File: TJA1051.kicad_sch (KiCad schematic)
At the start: 9 parts, among them U1 BMI088

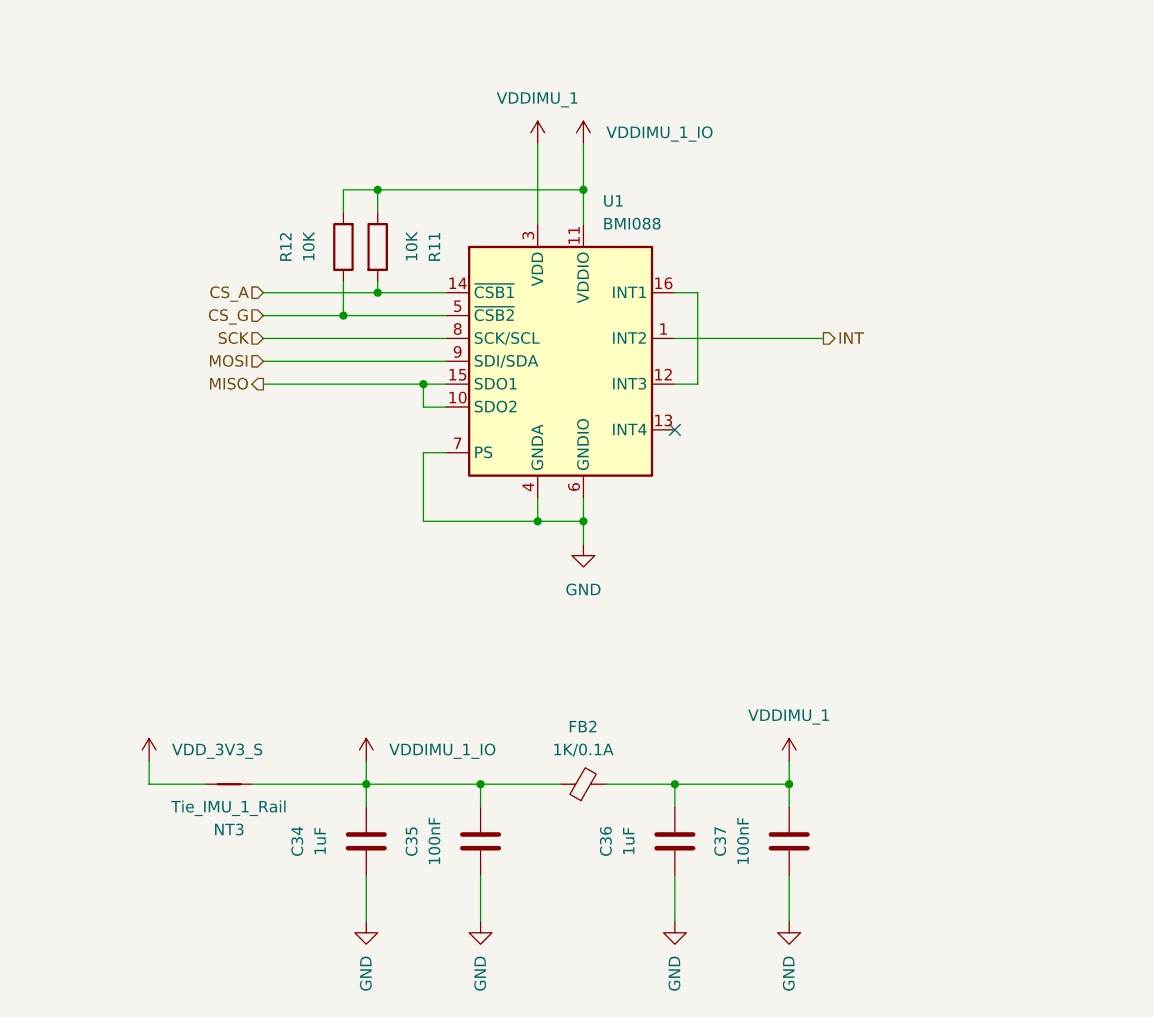
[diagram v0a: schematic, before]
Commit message: progress
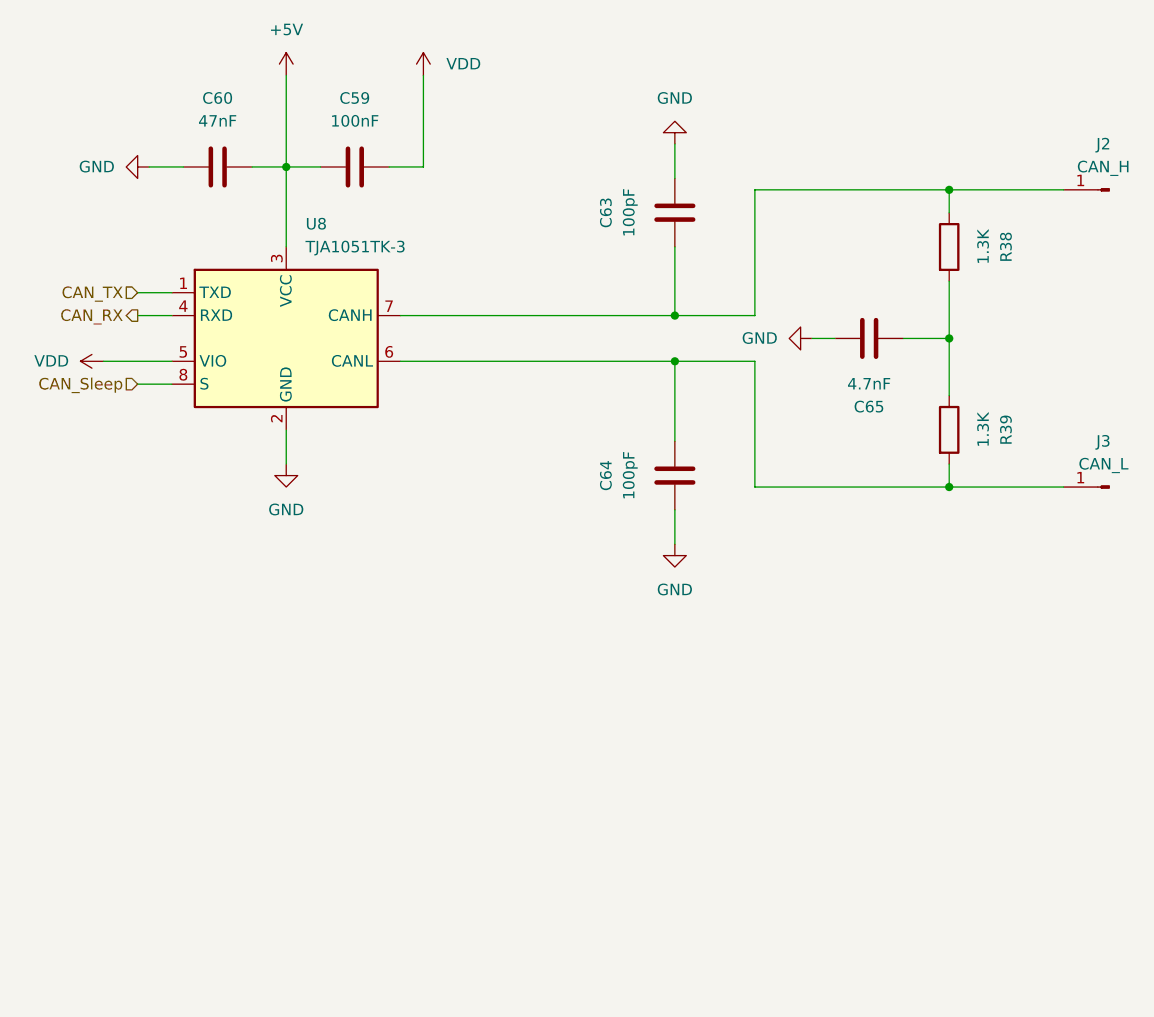
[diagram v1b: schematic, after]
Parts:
- removed C34, C36: 1uF, Capacitor_SMD:C_0805_2012Metric, symbol Device:C
- removed C35, C37: 100nF, Capacitor_SMD:C_0805_2012Metric, symbol Device:C
- removed FB2: 1K/0.1A, Inductor_SMD:L_0603_1608Metric, symbol Device:FerriteBead_Small
- removed NT3: Tie_IMU_1_Rail, NetTie:NetTie-2_SMD_Pad0.5mm, symbol Device:NetTie_2
- removed R11, R12: 10K, Resistor_SMD:R_0805_2012Metric, symbol Device:R
- removed U1: BMI088, Package_LGA:Bosch_LGA-16_4.5x3mm_P0.5mm_LayoutBorder7x1y_ClockwisePinNumbering, symbol Sensor_Motion:BMI088
- added C59: 100nF, Capacitor_SMD:C_0805_2012Metric, symbol Device:C
- added C60: 47nF, Capacitor_SMD:C_0805_2012Metric, symbol Device:C
- added C63, C64: 100pF, Capacitor_SMD:C_0805_2012Metric, symbol Device:C
- added C65: 4.7nF, Capacitor_SMD:C_0805_2012Metric, symbol Device:C
- added J2: CAN_H, Connector_Wire:SolderWirePad_1x01_SMD_1.5x3mm, symbol Connector:Conn_01x01_Pin
- added J3: CAN_L, Connector_Wire:SolderWirePad_1x01_SMD_1.5x3mm, symbol Connector:Conn_01x01_Pin
- added R38, R39: 1.3K, Resistor_SMD:R_0805_2012Metric, symbol Device:R
- added U8: TJA1051TK-3, Package_SON:HVSON-8-1EP_3x3mm_P0.65mm_EP1.6x2.4mm, symbol Interface_CAN_LIN:TJA1051TK-3
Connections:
- net GND: now also C60.2, C63.1, C64.2, C65.1, U8.2 (GND), U8.9 (GND)
- new net: C63.2, J2.1 (Pin_1), R38.1, U8.7 (CANH)
- new net: C65.2, R38.2, R39.1
- new net: C64.1, J3.1 (Pin_1), R39.2, U8.6 (CANL)
- new net +5V: C59.2, C60.1, U8.3 (VCC)
- new net CAN_RX: U8.4 (RXD)
- new net CAN_Sleep: U8.8 (S)
- new net CAN_TX: U8.1 (TXD)
- new net VDD: C59.1, U8.5 (VIO)
- no-connect marks 1 -> 0
